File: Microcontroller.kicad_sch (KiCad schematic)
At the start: 25 parts, among them J1 GT-USB-7010ASV, J5 B8B-PH-SM4-TB, SW2 KMR231NG, SW3 KMR231NG, U1 ESP32-S3-MINI-1

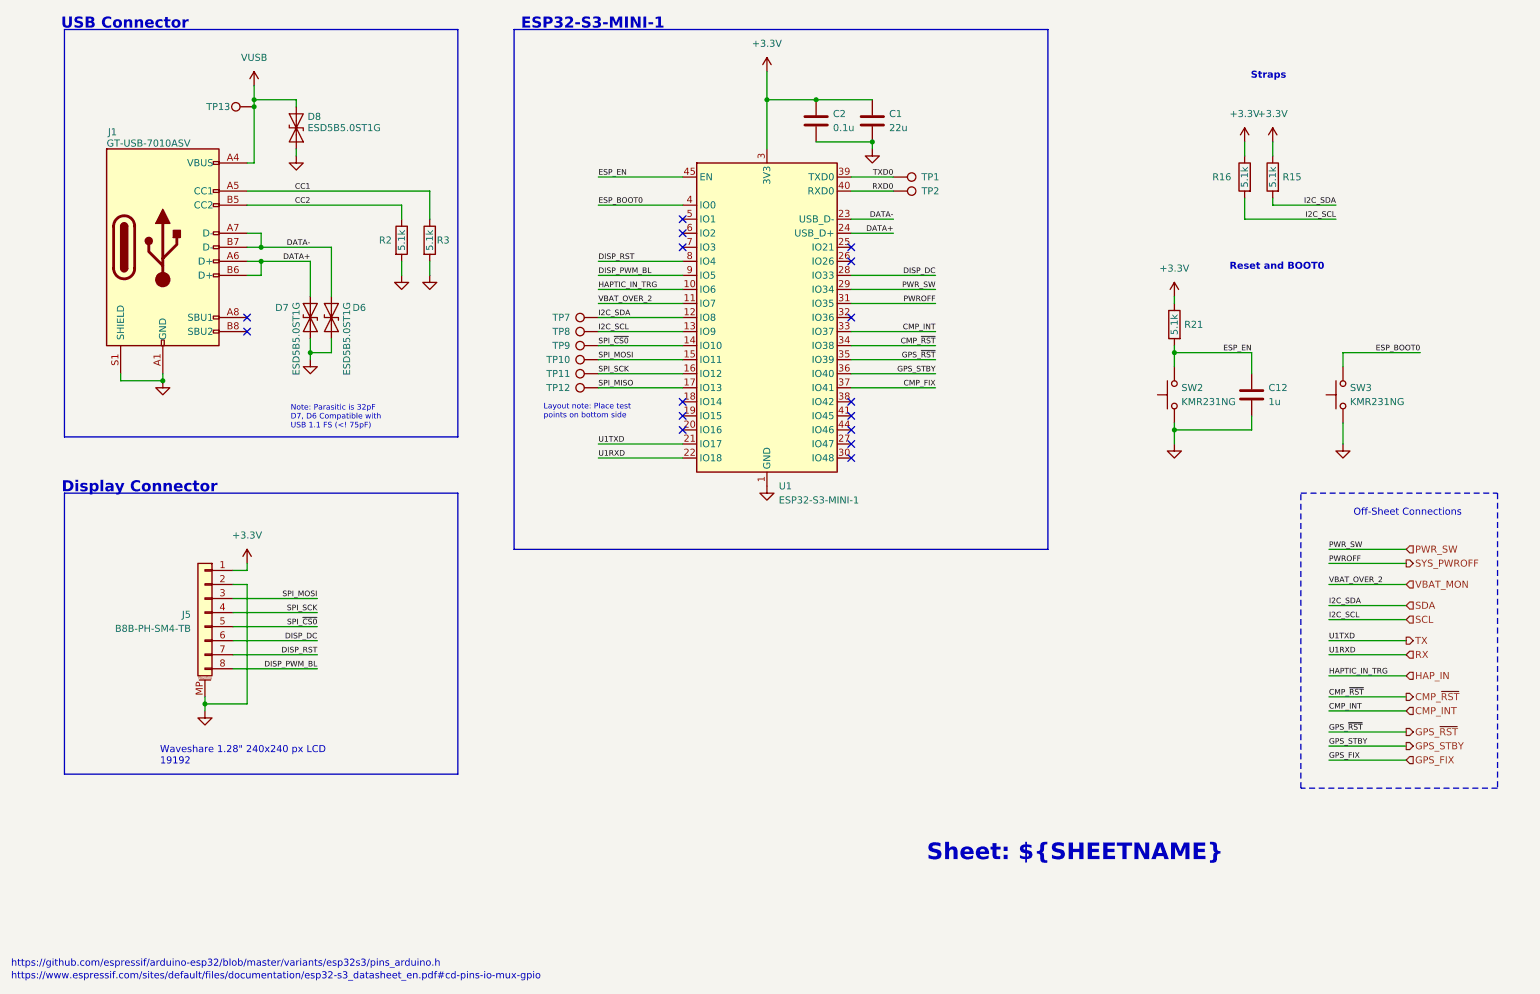
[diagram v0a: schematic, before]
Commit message: Lots of board layout
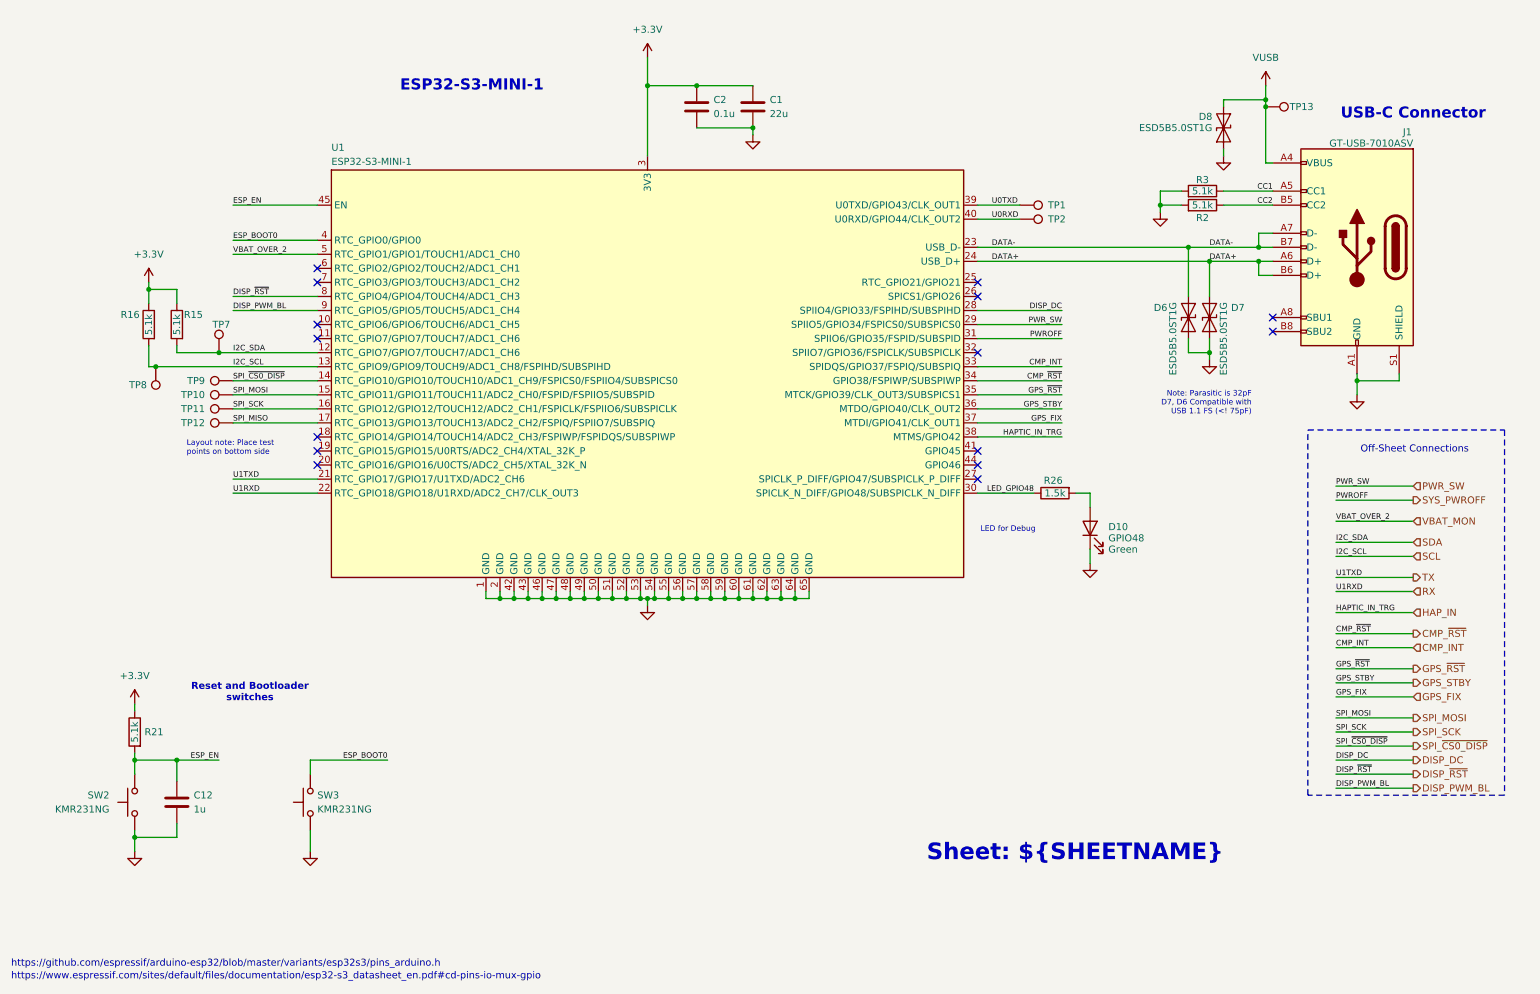
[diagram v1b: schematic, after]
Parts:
- removed J5: B8B-PH-SM4-TB, Connector_JST:JST_PH_B8B-PH-SM4-TB_1x08-1MP_P2.00mm_Vertical, symbol Connector_Generic_MountingPin:Conn_01x08_MountingPin
- removed U1: ESP32-S3-MINI-1, RF_Module:ESP32-S2-MINI-1, symbol RF_Module:ESP32-S3-MINI-1
- added D10: GPIO48, Diode_SMD:D_0603_1608Metric, symbol Device:LED
- added R26: 1.5k, Resistor_SMD:R_0603_1608Metric, symbol Device:R
- added U1: ESP32-S3-MINI-1, RF_Module:ESP32-S2-MINI-1, symbol RF_Module1:ESP32-S3-MINI-1
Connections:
- net +3.3V: now also U1.3 (3V3)
- net CMP_INT: now also U1.33 (SPIDQS/GPIO37/FSPIQ/SUBSPIQ)
- net CMP_~{RST}: now also U1.34 (GPIO38/FSPIWP/SUBSPIWP)
- net DATA+: now also U1.24 (USB_D+)
- net DATA-: now also U1.23 (USB_D-)
- net DISP_DC: now also U1.28 (SPIIO4/GPIO33/FSPIHD/SUBSPIHD)
- net DISP_PWM_BL: now also U1.9 (RTC_GPIO5/GPIO5/TOUCH5/ADC1_CH4)
- net ESP_BOOT0: now also U1.4 (RTC_GPIO0/GPIO0)
- net ESP_EN: now also U1.45 (EN)
- net GND: now also D10.1 (K), U1.1 (GND), U1.2 (GND), U1.42 (GND), U1.43 (GND), U1.46 (GND), U1.47 (GND), U1.48 (GND), U1.49 (GND), U1.50 (GND), U1.51 (GND), U1.52 (GND), U1.53 (GND), U1.54 (GND), U1.55 (GND), U1.56 (GND), U1.57 (GND), U1.58 (GND), U1.59 (GND), U1.60 (GND), U1.61 (GND), U1.62 (GND), U1.63 (GND), U1.64 (GND), U1.65 (GND)
- net GPS_FIX: now also U1.37 (MTDI/GPIO41/CLK_OUT1)
- net GPS_STBY: now also U1.36 (MTDO/GPIO40/CLK_OUT2)
- net GPS_~{RST}: now also U1.35 (MTCK/GPIO39/CLK_OUT3/SUBSPICS1)
- net HAP_IN: now also U1.38 (MTMS/GPIO42)
- net PWR_SW: now also U1.29 (SPIIO5/GPIO34/FSPICS0/SUBSPICS0)
- net RX: now also U1.22 (RTC_GPIO18/GPIO18/U1RXD/ADC2_CH7/CLK_OUT3)
- net SCL: now also U1.13 (RTC_GPIO9/GPIO9/TOUCH9/ADC1_CH8/FSPIHD/SUBSPIHD)
- net SDA: now also U1.12 (RTC_GPIO7/GPIO7/TOUCH7/ADC1_CH6)
- net SPI_MISO: now also U1.17 (RTC_GPIO13/GPIO13/TOUCH13/ADC2_CH2/FSPIQ/FSPIIO7/SUBSPIQ)
- net SPI_MOSI: now also U1.15 (RTC_GPIO11/GPIO11/TOUCH11/ADC2_CH0/FSPID/FSPIIO5/SUBSPID)
- net SPI_SCK: now also U1.16 (RTC_GPIO12/GPIO12/TOUCH12/ADC2_CH1/FSPICLK/FSPIIO6/SUBSPICLK)
- net SYS_PWROFF: now also U1.31 (SPIIO6/GPIO35/FSPID/SUBSPID)
- net TX: now also U1.21 (RTC_GPIO17/GPIO17/U1TXD/ADC2_CH6)
- net VBAT_MON: now also U1.5 (RTC_GPIO1/GPIO1/TOUCH1/ADC1_CH0)
- net RXD0 renamed U0RXD
- net U0RXD: now also U1.40 (U0RXD/GPIO44/CLK_OUT2)
- net SPI_~{CS0} renamed SPI_~{CS0_DISP}
- net SPI_~{CS0_DISP}: now also U1.14 (RTC_GPIO10/GPIO10/TOUCH10/ADC1_CH9/FSPICS0/FSPIIO4/SUBSPICS0)
- net TXD0 renamed U0TXD
- net U0TXD: now also U1.39 (U0TXD/GPIO43/CLK_OUT1)
- new net: D10.2 (A), R26.2
- new net DISP_~{RST}: U1.8 (RTC_GPIO4/GPIO4/TOUCH4/ADC1_CH3)
- new net LED_GPIO48: R26.1, U1.30 (SPICLK_N_DIFF/GPIO48/SUBSPICLK_N_DIFF)
- no-connect marks 16 -> 15
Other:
- note added: "LED for Debug"
- note added: "Reset and Bootloader switches"
- note added: "USB-C Connector"
- note removed: "Display Connector"
- note removed: "Reset and BOOT0"
- note removed: "Straps"
- note removed: "USB Connector"
- note removed: "Waveshare 1.28" 240x240 px LCD 19192"
- moved on the sheet: C1, C12, C2, D6, D7, D8, J1, R15, R16, R2, R21, R3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
